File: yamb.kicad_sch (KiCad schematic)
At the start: 14 parts, among them J1 Barrel_Jack, J2 I2C, J3 HEADER, J4 HEADER_2.54, J5 Remote_Reset, J6 Power_Switch, P1 USB_C_Plug_USB2.0, SW1 RESET, U1 TPS3808DBV, U2 MCSBC, U3 SVR, U4 RAK4630

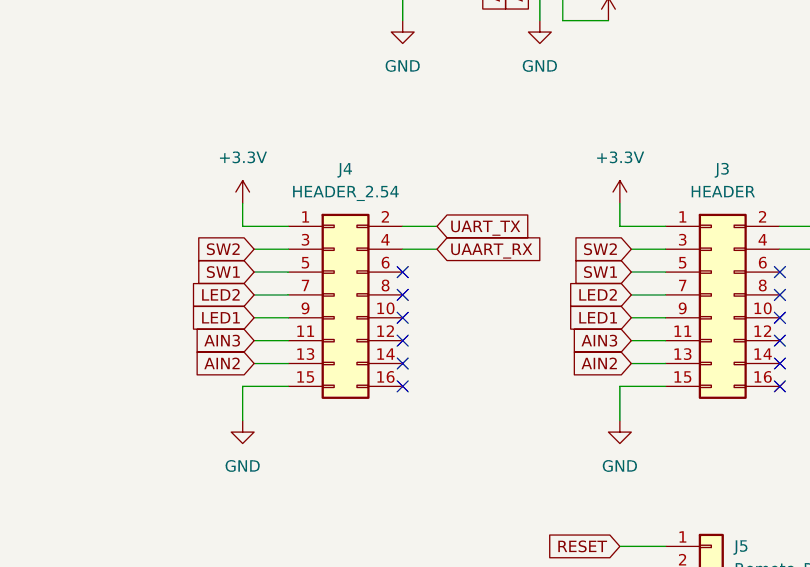
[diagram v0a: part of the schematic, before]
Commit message: PCB layout first pass
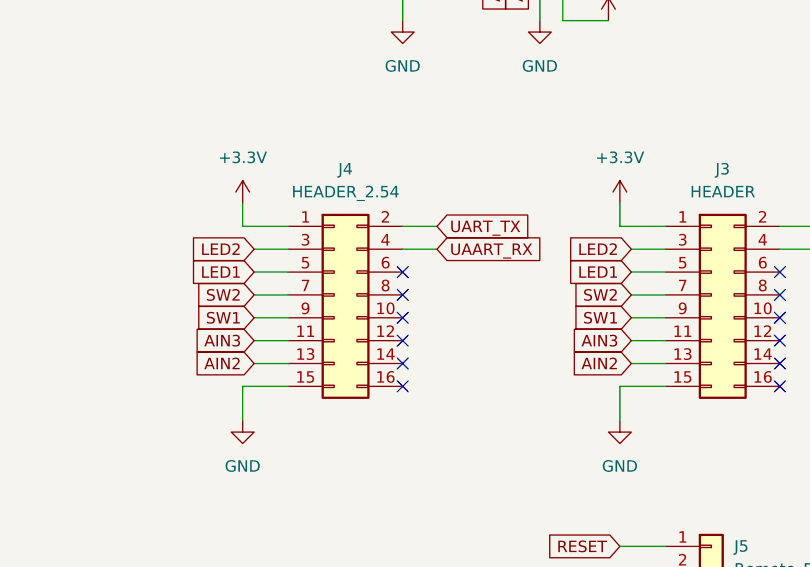
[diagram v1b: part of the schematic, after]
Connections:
- net LED1: now also J3.5 (Pin_5), J4.5 (Pin_5); no longer J3.9 (Pin_9), J4.9 (Pin_9)
- net LED2: now also J3.3 (Pin_3), J4.3 (Pin_3); no longer J3.7 (Pin_7), J4.7 (Pin_7)
- net SW1: now also J3.9 (Pin_9), J4.9 (Pin_9); no longer J3.5 (Pin_5), J4.5 (Pin_5)
- net SW2: now also J3.7 (Pin_7), J4.7 (Pin_7); no longer J3.3 (Pin_3), J4.3 (Pin_3)
